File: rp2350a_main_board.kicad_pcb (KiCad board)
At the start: 2 copper layers, 61 x 45.7 mm, 65 parts, among them J1 USB_C_Receptacle_USB2.0_16P, J2 Micro_SD_Card_Det1, J3 Conn_02x10_Odd_Even, J4 SM03B-SRSS-TB, J5 SM03B-SRSS-TB, J6 Conn_02x10_Odd_Even, SW1 SW_Push, SW2 SW_Push, U1 RP2350_60QFN, U2 W25Q16JVSS, U3 APS1604M-3SQRx-SN, U4 AP2112K-3.3, Y1 ABM8-272-T3

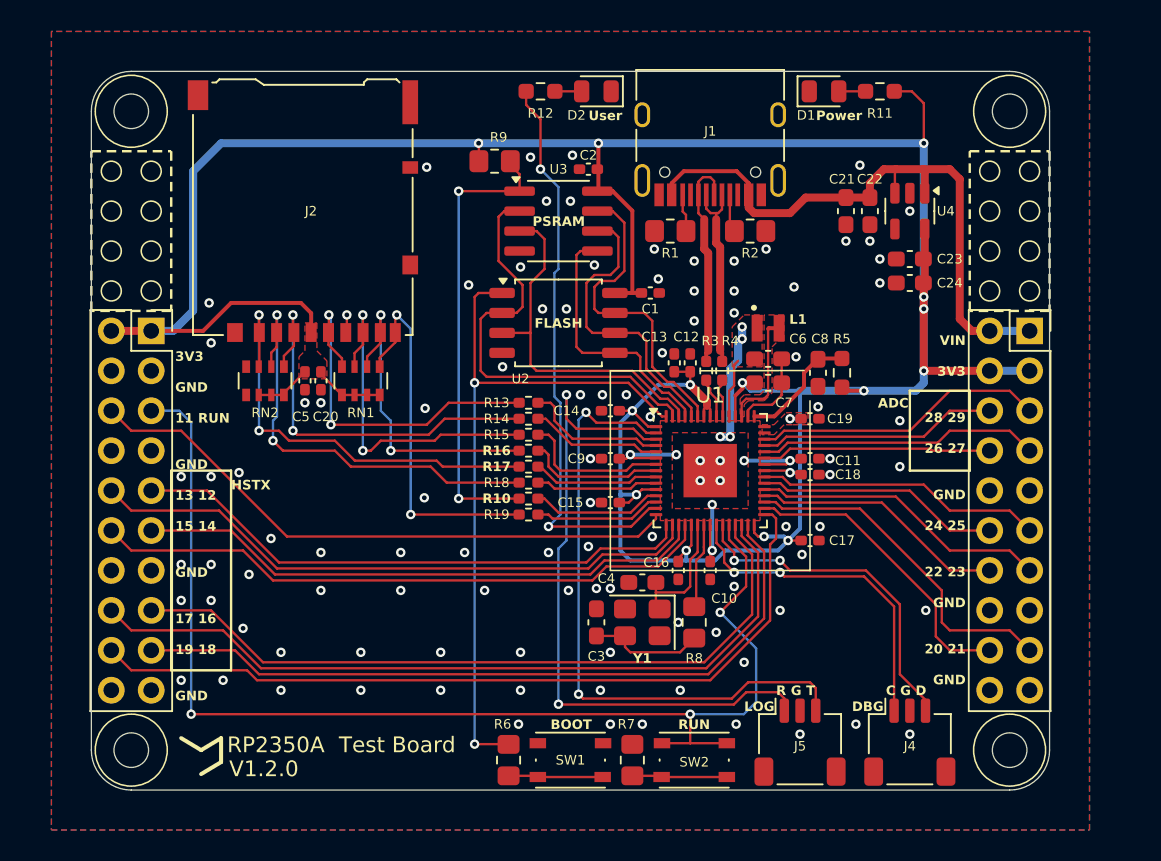
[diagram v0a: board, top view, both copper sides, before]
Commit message: V1.0.0
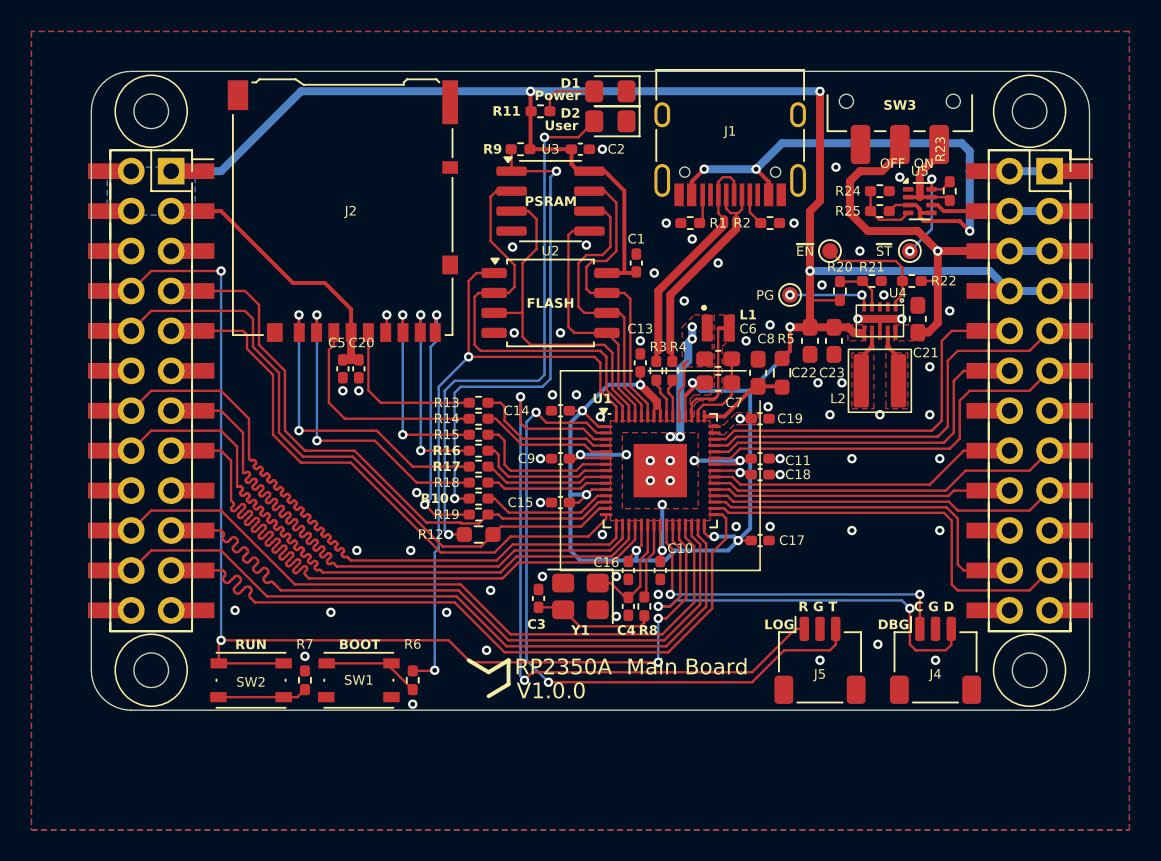
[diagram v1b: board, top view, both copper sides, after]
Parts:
- removed C12: 100n, Capacitor_SMD:C_0402_1005Metric_Pad0.74x0.62mm_HandSolder
- removed C24: 10u, Capacitor_SMD:C_0603_1608Metric_Pad1.08x0.95mm_HandSolder
- removed RN1, RN2: 10k, Resistor_SMD:R_Array_Convex_4x0603
- added J7: Conn_02x12, Connector_PinSocket_2.54mm:PinSocket_2x12_P2.54mm_Vertical_SMD, F.Cu at (29.2, 45.7)
- added J8: Conn_02x12, Connector_PinSocket_2.54mm:PinSocket_2x12_P2.54mm_Vertical_SMD, F.Cu at (85.1, 45.7)
- added L2: 470n, Library:Inductor_SMD_L_4.0x4.0_H1.5, F.Cu at (75.6, 45.1)
- added R20: 511k, Resistor_SMD:R_0402_1005Metric_Pad0.72x0.64mm_HandSolder, F.Cu at (73.0, 39.4)
- added R21: 91k, Resistor_SMD:R_0402_1005Metric_Pad0.72x0.64mm_HandSolder, F.Cu at (75.1, 38.7)
- added R22: 10k, Resistor_SMD:R_0402_1005Metric_Pad0.72x0.64mm_HandSolder, F.Cu at (77.6, 38.7)
- added R23: 10k, Resistor_SMD:R_0402_1005Metric_Pad0.72x0.64mm_HandSolder, F.Cu at (80.0, 33.0)
- added R24: 10k, Resistor_SMD:R_0402_1005Metric_Pad0.72x0.64mm_HandSolder, F.Cu at (75.6, 33.0)
- added R25: 33k, Resistor_SMD:R_0402_1005Metric_Pad0.72x0.64mm_HandSolder, F.Cu at (75.6, 34.3)
- added SW3: SW_SPDT, Button_Switch_SMD:SW_SPDT_CK_JS102011SAQN, F.Cu at (76.8, 27.3)
- added TP1: ST, TestPoint:TestPoint_Pad_D1.0mm, F.Cu at (77.5, 36.8)
- added TP2: EN, TestPoint:TestPoint_Pad_D1.0mm, F.Cu at (72.4, 36.8)
- added TP4: PG, TestPoint:TestPoint_Pad_D1.0mm, F.Cu at (69.8, 39.6)
- added U5: TPS2116DRL, Package_TO_SOT_SMD:SOT-583-8, F.Cu at (78.1, 33.7)
- C3, C4: footprint Capacitor_SMD:C_0603_1608Metric_Pad1.08x0.95mm_HandSolder -> Capacitor_SMD:C_0402_1005Metric_Pad0.74x0.62mm_HandSolder
- D1, D2: footprint LED_SMD:LED_0805_2012Metric -> LED_SMD:LED_0805_2012Metric_Pad1.15x1.40mm_HandSolder
- J3, J6: value Conn_02x10_Odd_Even -> Conn_02x12; footprint Connector_PinSocket_2.54mm:PinSocket_2x10_P2.54mm_Vertical -> Connector_PinSocket_2.54mm:PinSocket_2x12_P2.54mm_Vertical
- R1, R2, R6, R7, R8, R9: footprint Resistor_SMD:R_0805_2012Metric_Pad1.20x1.40mm_HandSolder -> Resistor_SMD:R_0402_1005Metric_Pad0.72x0.64mm_HandSolder
- R11: value 470 -> 1k; footprint Resistor_SMD:R_0603_1608Metric_Pad0.98x0.95mm_HandSolder -> Resistor_SMD:R_0402_1005Metric_Pad0.72x0.64mm_HandSolder
- U4: value AP2112K-3.3 -> TPS63802; footprint Package_TO_SOT_SMD:SOT-23-5 -> Library:TPS63802
- moved J6 58.0 mm to (86.4, 31.8)
- moved J3 55.5 mm to (30.5, 31.8)
- moved SW2 28.6 mm to (35.6, 64.1)
- moved R12 28.5 mm to (50.0, 54.9), turned to 180 degrees
- moved R11 21.6 mm to (54.0, 27.9), turned to 0 degrees
- moved R7 21.4 mm to (39.0, 64.1)
- moved SW1 14.4 mm to (42.4, 64.1), turned to 180 degrees
- moved D1 13.6 mm to (58.4, 26.7), turned to 180 degrees
- moved C22 9.09 mm to (71.1, 42.5)
- moved C21 8.24 mm to (78.0, 41.1), turned to 90 degrees
- moved R6 7.94 mm to (45.8, 64.1)
- moved U4 7.24 mm to (75.6, 41.3)
- moved C23 7.10 mm to (72.6, 42.5), turned to -90 degrees
- moved J4 5.46 mm to (79.1, 62.9)
- moved J5 5.36 mm to (71.8, 62.9)
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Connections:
- C21 pad 1: VBUS -> VIN
- C22 pad 1: VBUS -> +3V3
- J1 pad A4: VBUS -> VUSB
- J1 pad A9: VBUS -> VUSB
- J1 pad B4: VBUS -> VUSB
- J1 pad B9: VBUS -> VUSB
- J3 pad 1: VBUS -> +3V3
- J3 pad 10: GND -> /GPIO10
- J3 pad 11: /GPIO25 -> GND
- J3 pad 12: /GPIO24 -> GND
- J3 pad 13: /GPIO23 -> /GPIO13
- J3 pad 14: /GPIO22 -> /GPIO12
- J3 pad 15: GND -> /GPIO15
- J3 pad 16: GND -> /GPIO14
- J3 pad 17: /GPIO21 -> GND
- J3 pad 18: /GPIO20 -> GND
- J3 pad 19: GND -> /GPIO17
- J3 pad 2: VBUS -> +3V3
- J3 pad 20: GND -> /GPIO16
- J3 pad 5: /GPIO29_ADC3 -> GND
- J3 pad 6: /GPIO28_ADC2 -> GND
- J3 pad 7: /GPIO27_ADC1 -> /GPIO9
- J3 pad 8: /GPIO26_ADC0 -> /RUN
- J3 pad 9: GND -> /GPIO11
- J6 pad 1: +3V3 -> VUSB
- J6 pad 10: /GPIO13 -> /GPIO29_ADC3
- J6 pad 11: /GPIO14 -> /GPIO26_ADC0
- J6 pad 12: /GPIO15 -> /GPIO27_ADC1
- J6 pad 15: /GPIO16 -> /GPIO24
- J6 pad 16: /GPIO17 -> /GPIO25
- J6 pad 17: /GPIO18 -> /GPIO22
- J6 pad 18: /GPIO19 -> /GPIO23
- J6 pad 2: +3V3 -> VUSB
- J6 pad 3: GND -> VBAT
- J6 pad 4: GND -> VBAT
- J6 pad 5: /RUN -> VIN
- J6 pad 6: /GPIO11 -> VIN
- J6 pad 7: GND -> +3V3
- J6 pad 8: GND -> +3V3
- J6 pad 9: /GPIO12 -> /GPIO28_ADC2
- U1 pad 15: GND -> /GPIO11
- U1 pad 17: GND -> /GPIO13
- U1 pad 19: GND -> /GPIO15
- U1 pad 28: GND -> /GPIO17
- U1 pad 31: GND -> /GPIO19
- U4 pad 1: VBUS -> Net-(U4-EN)
- U4 pad 3: VBUS -> GND
- U4 pad 4: unconnected-(U4-NC-Pad4) -> Net-(U4-FB)
- U4 pad 5: +3V3 -> Net-(U4-PG)
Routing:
- net VBUS: track 40.1 -> 0.00 mm
- net VUSB: track 0.00 -> 38.9 mm, vias 0 -> 3
- net Net-(D2-A): track 1.87 -> 35.7 mm, vias 0 -> 2
- net /GPIO9: track 8.05 -> 37.0 mm
- net VIN: track 0.00 -> 26.1 mm, vias 0 -> 1
- net +3V3: track 205.5 -> 186.9 mm, vias 16 -> 13
- net /SD_CLK: track 23.2 -> 10.5 mm, vias 2 -> 0
- net /SD_CMD: track 25.9 -> 14.0 mm, vias 2 -> 0
- net /GPIO28_ADC2: track 15.2 -> 26.8 mm
- net /GPIO26_ADC0: track 14.6 -> 25.0 mm
- net /GPIO12: track 36.1 -> 46.0 mm
- net /SD_D0: track 22.5 -> 13.0 mm
- net /GPIO14: track 36.6 -> 46.1 mm
- net /GPIO15: track 39.9 -> 48.7 mm
- net /SD_D3/CD: track 28.3 -> 19.9 mm
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- added copper zone on B.Cu, net +3V3
- added copper zone on F.Cu, net /PS_L1
- added copper zone on F.Cu, net /PS_L2
- added copper zone on F.Cu, net VIN
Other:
- board size 61 x 45.7 mm -> 63.5 x 40.6 mm
- board text added: "Main Board"
- board text added: "OFF ON"
- board text added: "ON OFF"
- board text added: "PG"
- board text added: "RP2350A Main Board"
- board text added: "USB"
- board text added: "V1.0.0"
- board text added: "microSD"
- board text added: "~{EN}"
- board text added: "~{ST}"
- board text removed: "3V3 GND 11 RUN GND 13 12 15 14 GND 17 16 19 18 GND"
- board text removed: "ADC"
- board text removed: "HSTX"
- board text removed: "Test Board"
- board text removed: "V1.2.0"
- board text removed: "VIN 3V3 28 29 26 27 GND 24 25 22 23 GND 20 21 GND"
